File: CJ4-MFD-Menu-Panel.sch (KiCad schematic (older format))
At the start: 50 parts, among them SW1 SW_Push_LED, SW10 5_Way_Switch, SW11 SW_Push_LED, SW12 SW_Push_LED, SW13 SW_Push_LED, SW14 SW_Push_LED, SW15 SW_Push_LED, SW16 SW_Push_LED, SW17 SW_Push_LED, SW18 SW_Push_LED, SW19 SW_Push_LED, SW2 SW_Push_LED, SW20 SW_Push_LED, SW21 SW_Push_LED, SW3 SW_Push_LED, SW4 SW_Push_LED, SW5 SW_Push_LED, SW6 SW_Push_LED, SW7 SW_Push_LED, SW8 SW_Push_LED, SW9 SW_Push_LED, U1 MCP23017_SO, U2 MCP23017_SO, U3 IS31FL3733B

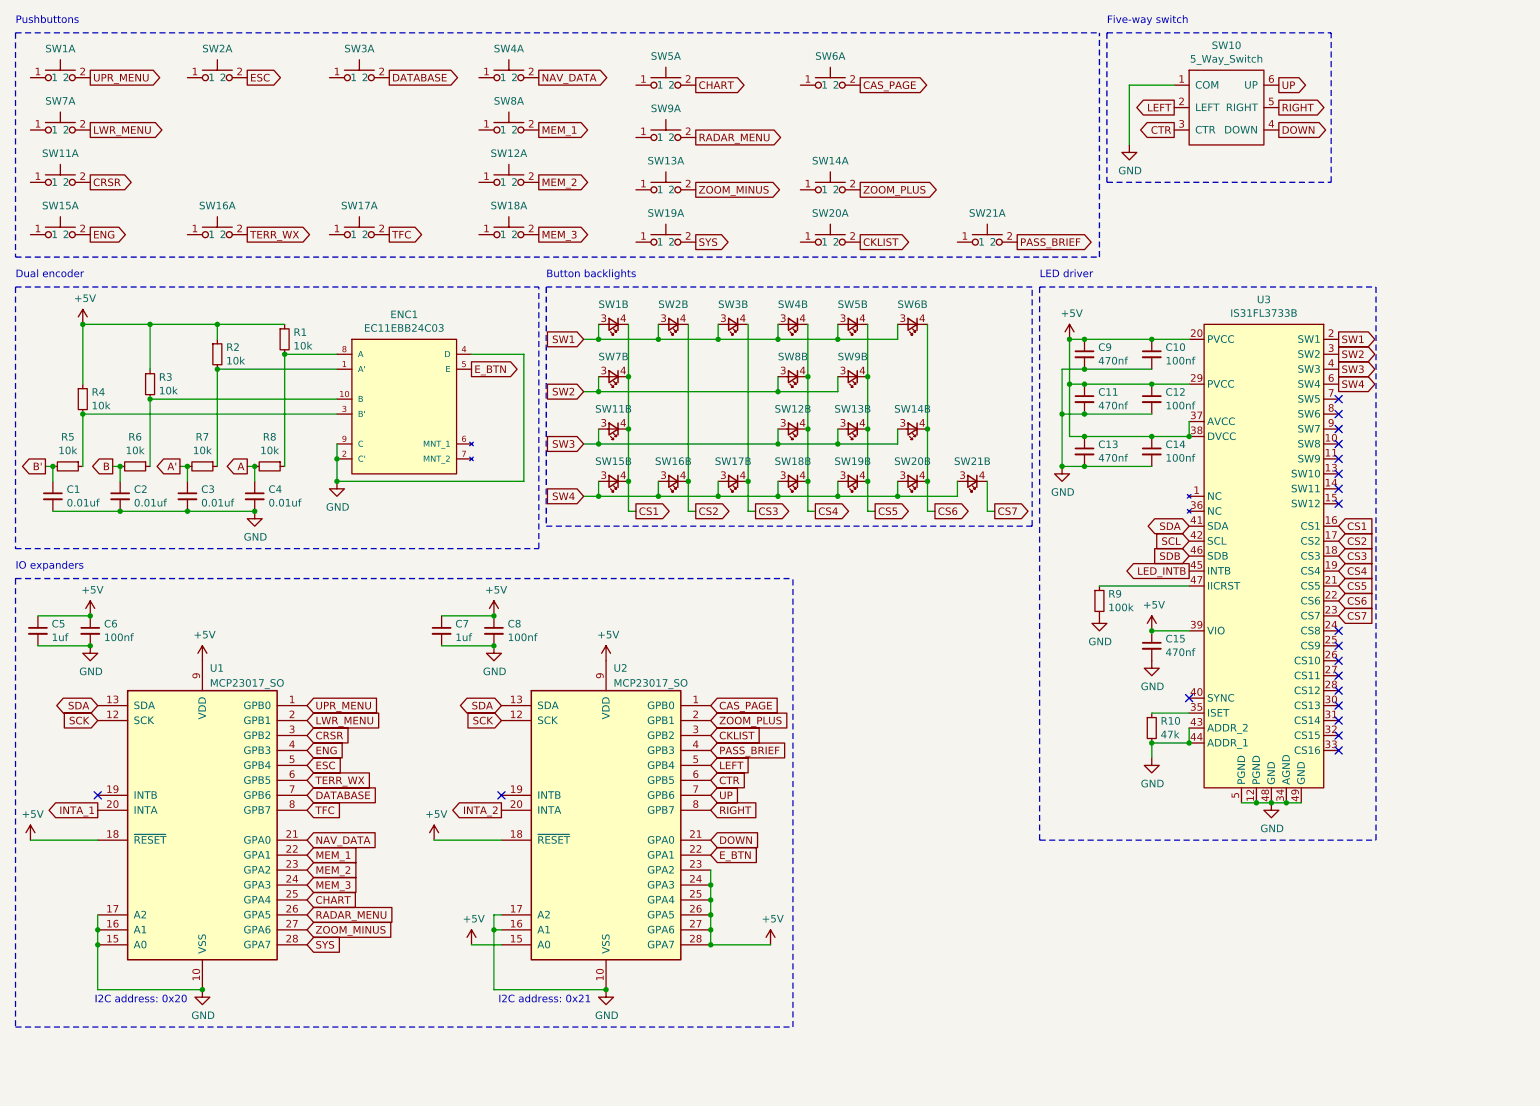
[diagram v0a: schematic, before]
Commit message: Layout + PCB
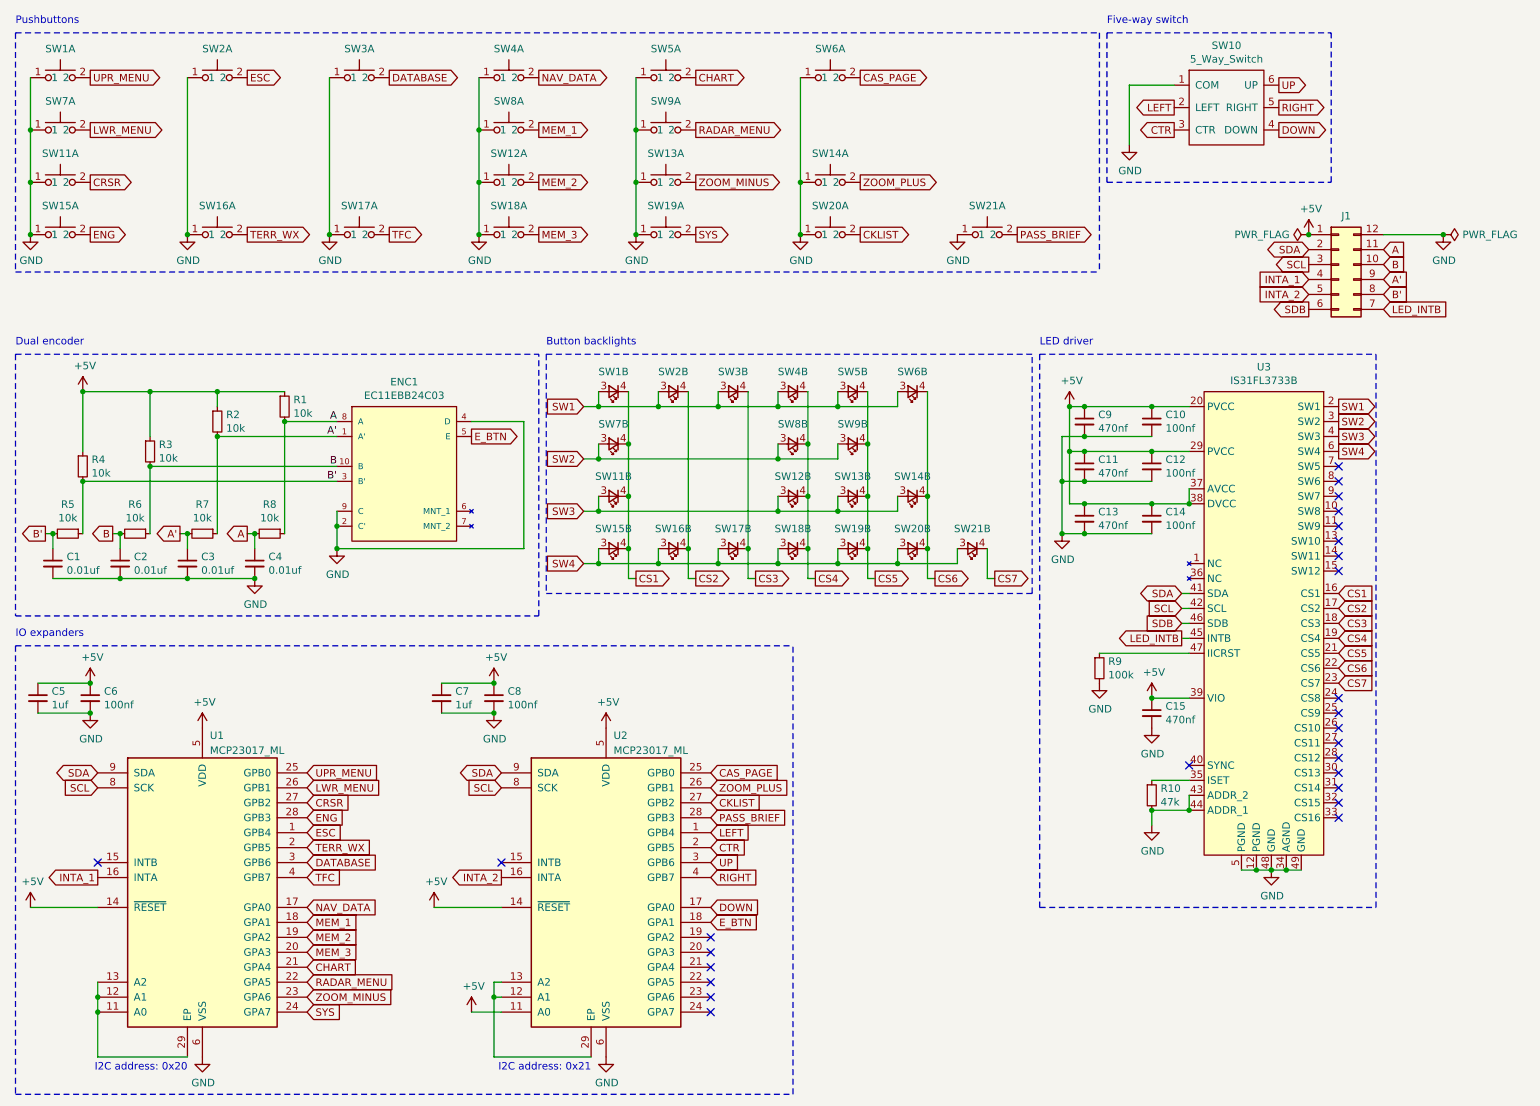
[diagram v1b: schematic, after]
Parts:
- removed U1, U2: MCP23017_SO, Package_SO:SOIC-28W_7.5x17.9mm_P1.27mm, symbol Interface_Expansion:MCP23017_SO
- added J1: Conn_02x06_Counter_Clockwise, Connector_PinHeader_2.54mm:PinHeader_2x06_P2.54mm_Vertical, symbol Connector_Generic:Conn_02x06_Counter_Clockwise
- added U1, U2: MCP23017_ML, Package_DFN_QFN:QFN-28-1EP_6x6mm_P0.65mm_EP4.25x4.25mm, symbol Interface_Expansion:MCP23017_ML
- C1, C10, C11, C12, C13, C14, C15, C2, C3, C4, C5, C6, C7, C8, C9, R1, R10, R2, R3, R4, R5, R6, R7, R8, R9: footprint (none) -> CJ4-MFD-Menu-Panel:Perfect_0402
- ENC1: footprint ALPS-EC11EBB24C03-* -> CJ4-MFD-Menu-Panel:ALPS-EC11EBB24C03-0
- SW1, SW11, SW12, SW13, SW14, SW15, SW16, SW17, SW18, SW19, SW2, SW20, SW21, SW3, SW4, SW5, SW6, SW7, SW8, SW9: footprint (none) -> CJ4-MFD-Menu-Panel:SW_PUSH_6mm
- SW10: footprint (none) -> CJ4-MFD-Menu-Panel:5_Way_Switch
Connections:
- net +5V: now also J1.1 (Pin_1), U1.14 (~RESET~), U1.5 (VDD), U2.11 (A0), U2.14 (~RESET~), U2.5 (VDD)
- net A: now also ENC1.8 (A), R1.2, R8.1, J1.11 (Pin_11)
- net A': now also ENC1.1 (A'), R2.2, R7.1, J1.9 (Pin_9)
- net B: now also ENC1.10 (B), R3.2, R6.1, J1.10 (Pin_10)
- net B': now also ENC1.3 (B'), R4.2, R5.1, J1.8 (Pin_8)
- net CAS_PAGE: now also U2.25 (GPB0)
- net CHART: now also U1.21 (GPA4)
- net CKLIST: now also U2.27 (GPB2)
- net CRSR: now also U1.27 (GPB2)
- net CTR: now also U2.2 (GPB5)
- net DATABASE: now also U1.3 (GPB6)
- net DOWN: now also U2.17 (GPA0)
- net ENG: now also U1.28 (GPB3)
- net ESC: now also U1.1 (GPB4)
- net E_BTN: now also U2.18 (GPA1)
- net GND: now also SW1.1, SW11.1, SW12.1, SW13.1, SW14.1, SW15.1, SW16.1, SW17.1, SW18.1, SW19.1, SW2.1, SW20.1, SW21.1, SW3.1, SW4.1, SW5.1, SW6.1, SW7.1, SW8.1, SW9.1, J1.12 (Pin_12), U1.6 (VSS), U2.6 (VSS)
- net INTA_1: now also J1.4 (Pin_4), U1.16 (INTA)
- net INTA_2: now also J1.5 (Pin_5), U2.16 (INTA)
- net LED_INTB: now also J1.7 (Pin_7)
- net LEFT: now also U2.1 (GPB4)
- net LWR_MENU: now also U1.26 (GPB1)
- net MEM_1: now also U1.18 (GPA1)
- net MEM_2: now also U1.19 (GPA2)
- net MEM_3: now also U1.20 (GPA3)
- net NAV_DATA: now also U1.17 (GPA0)
- net PASS_BRIEF: now also U2.28 (GPB3)
- net RADAR_MENU: now also U1.22 (GPA5)
- net RIGHT: now also U2.4 (GPB7)
- net SCL: now also J1.3 (Pin_3), U1.8 (SCK), U2.8 (SCK)
- net SDA: now also J1.2 (Pin_2), U1.9 (SDA), U2.9 (SDA)
- net SDB: now also J1.6 (Pin_6)
- net SYS: now also U1.24 (GPA7)
- net TERR_WX: now also U1.2 (GPB5)
- net TFC: now also U1.4 (GPB7)
- net UP: now also U2.3 (GPB6)
- net UPR_MENU: now also U1.25 (GPB0)
- net ZOOM_MINUS: now also U1.23 (GPA6)
- net ZOOM_PLUS: now also U2.26 (GPB1)
- new net: U1.11 (A0), U1.12 (A1), U1.13 (A2), U1.29 (EP)
- new net: U2.12 (A1), U2.13 (A2), U2.29 (EP)
- no-connect marks 20 -> 26
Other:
- moved on the sheet: C1, C10, C11, C12, C13, C14, C15, C2, C3, C4, C5, C6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
